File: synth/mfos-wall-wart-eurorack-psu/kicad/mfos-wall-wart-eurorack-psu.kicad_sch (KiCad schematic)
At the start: 43 parts, among them J1 JST-5, J2 TERMINAL-4, U1 L7812CV, U2 L7805CV, U3 L7912CV

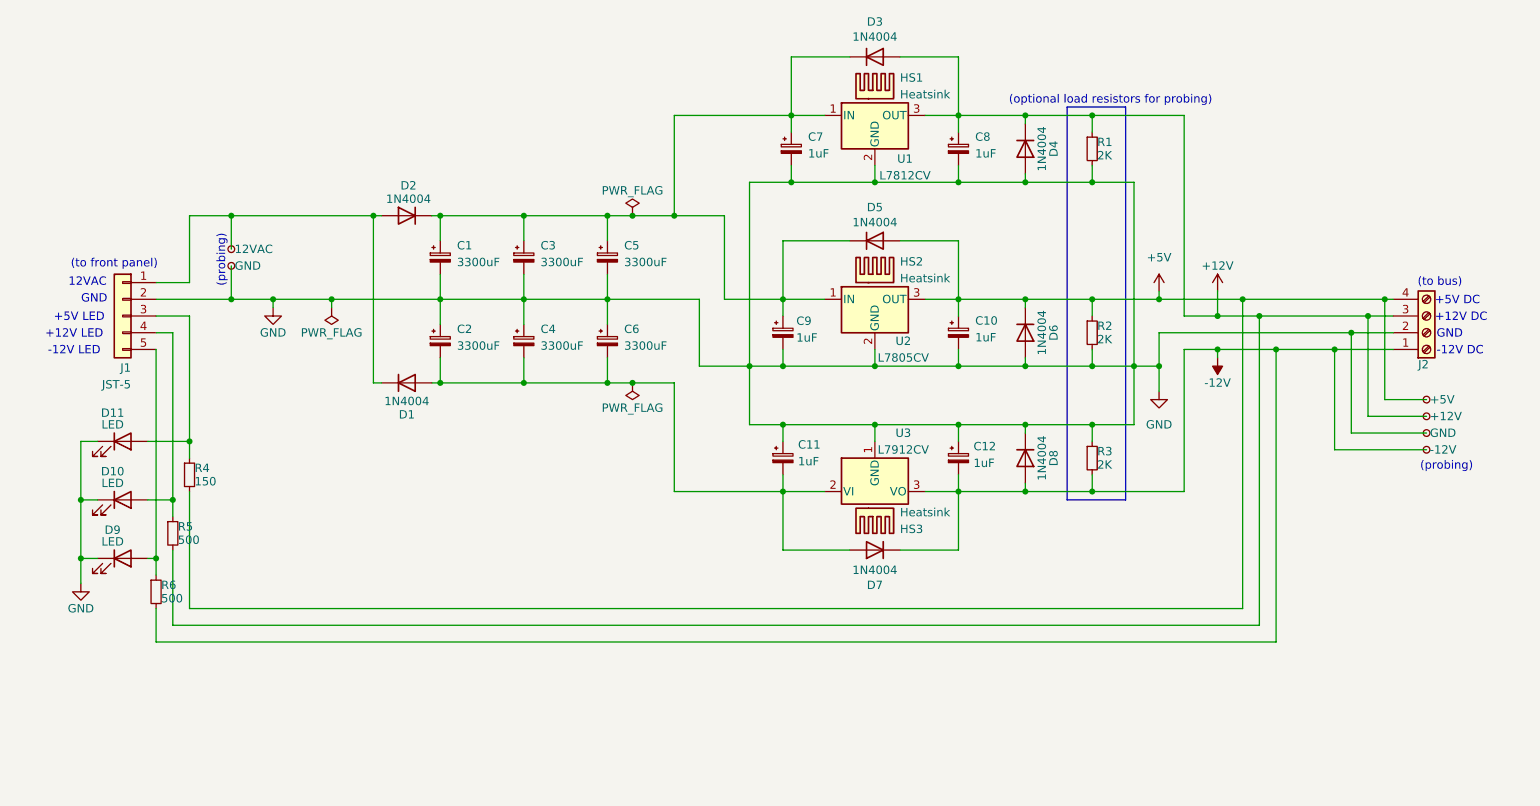
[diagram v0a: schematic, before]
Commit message: rev2
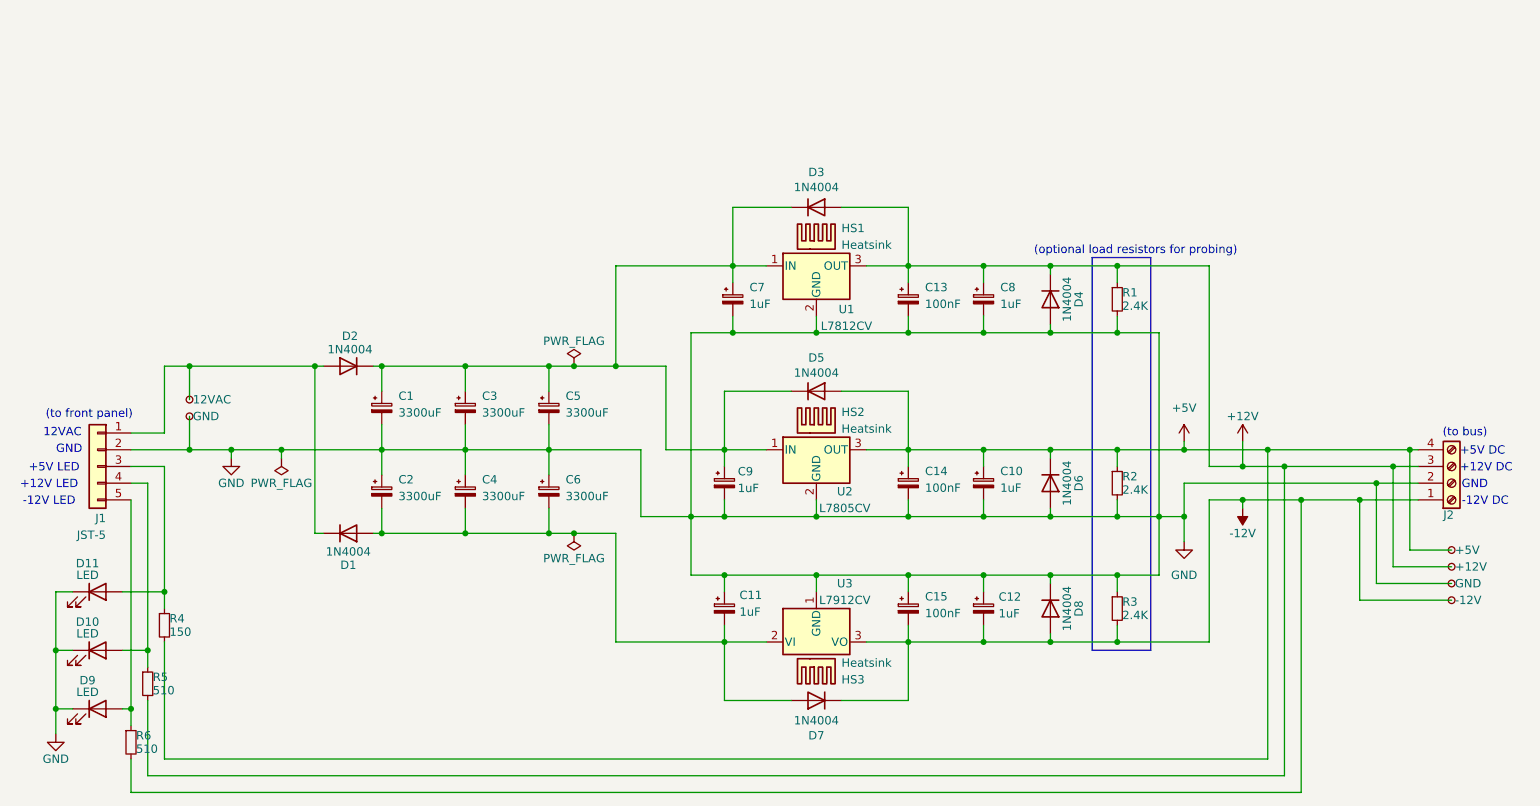
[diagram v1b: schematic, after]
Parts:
- added C13, C14, C15: 100nF, Capacitor_THT:C_Disc_D3.0mm_W2.0mm_P2.50mm, symbol Device:C_Polarized_Small
- C10, C11, C12, C7, C8, C9: footprint Capacitor_THT:CP_Radial_Tantal_D5.0mm_P2.50mm -> Capacitor_THT:CP_Radial_D5.0mm_P2.50mm
- J2: URL ?? -> https://www.amazon.com/gp/product/B0CFYHDC7L/ref=ppx_yo_dt_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
- R1, R2, R3: value 2K -> 2.4K; URL https://www.taydaelectronics.com/10-x-resistor-2k-ohm-1-2w-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 -> https://www.taydaelectronics.com/resistors/1-4w-metal-film-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
- R4: URL ?? -> https://www.taydaelectronics.com/resistors/1-4w-metal-film-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
- R5, R6: value 500 -> 510; URL ?? -> https://www.taydaelectronics.com/resistors/1-4w-metal-film-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
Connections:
- net +12V: now also C13.1
- net +5V: now also C14.1
- net -12V: now also C15.2
- net GND: now also C13.2, C14.2, C15.1
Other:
- note removed: "(probing)"
- moved on the sheet: C1, C10, C11, C12, C2, C3, C4, C5, C6, C7, C8, C9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
